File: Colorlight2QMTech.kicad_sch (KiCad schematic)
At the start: 16 parts, among them CN1 1473005-4, J1 Conn_02x32_Odd_Even, J2 Conn_02x32_Odd_Even, J3 Connector_USB_C_Receptacle_US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, J4-GND1 Conn_01x01_Male, SW1 TS-1187A-B-A-B, U1 AMS1117-3.3

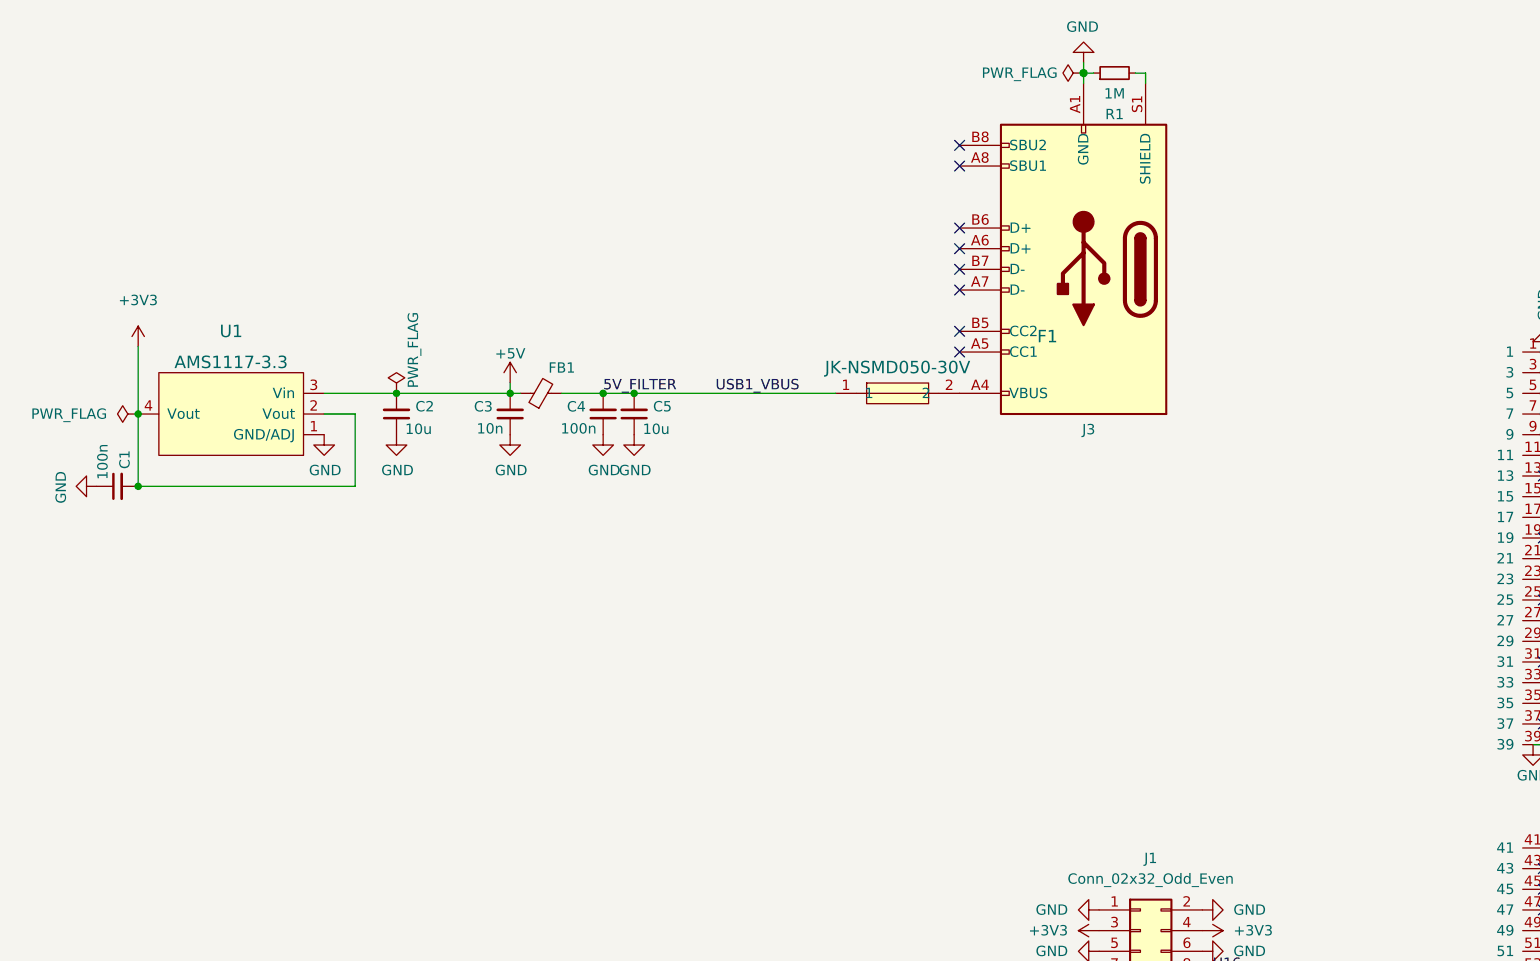
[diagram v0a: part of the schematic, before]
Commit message: tidy schematic and export
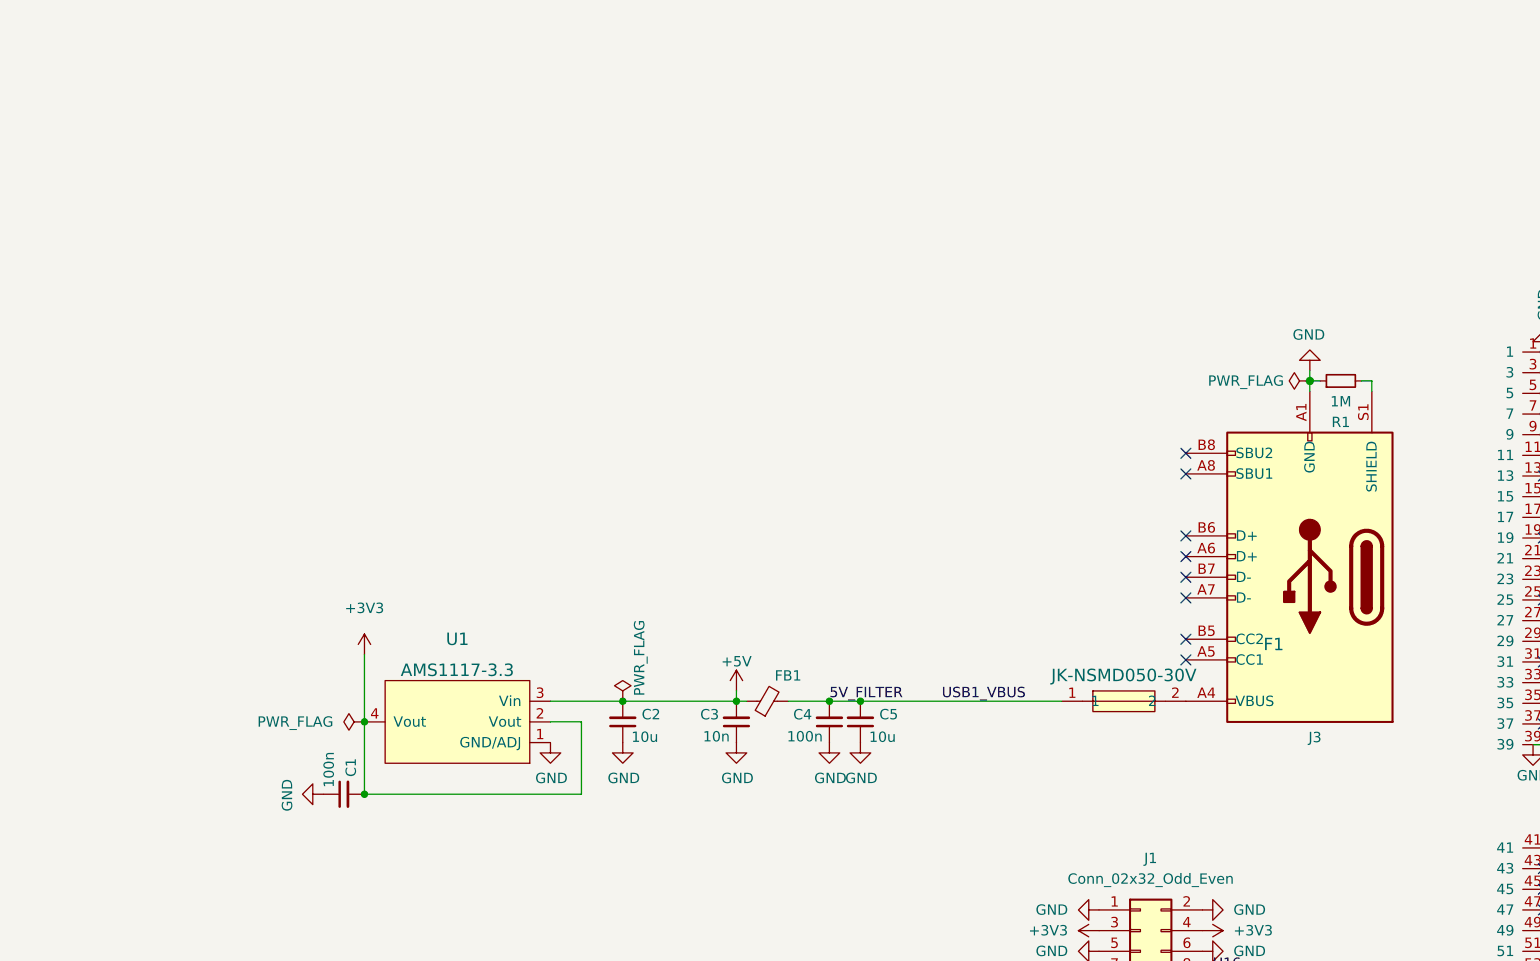
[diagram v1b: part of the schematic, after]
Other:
- moved on the sheet: C1, C2, C3, C4, C5, F1, FB1, J3, R1, U1
